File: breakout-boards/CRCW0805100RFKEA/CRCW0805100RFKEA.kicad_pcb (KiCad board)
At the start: 2 copper layers, 21.5 x 38.2 mm, 16 parts, among them J1 Conn_01x12, J2 Conn_01x12

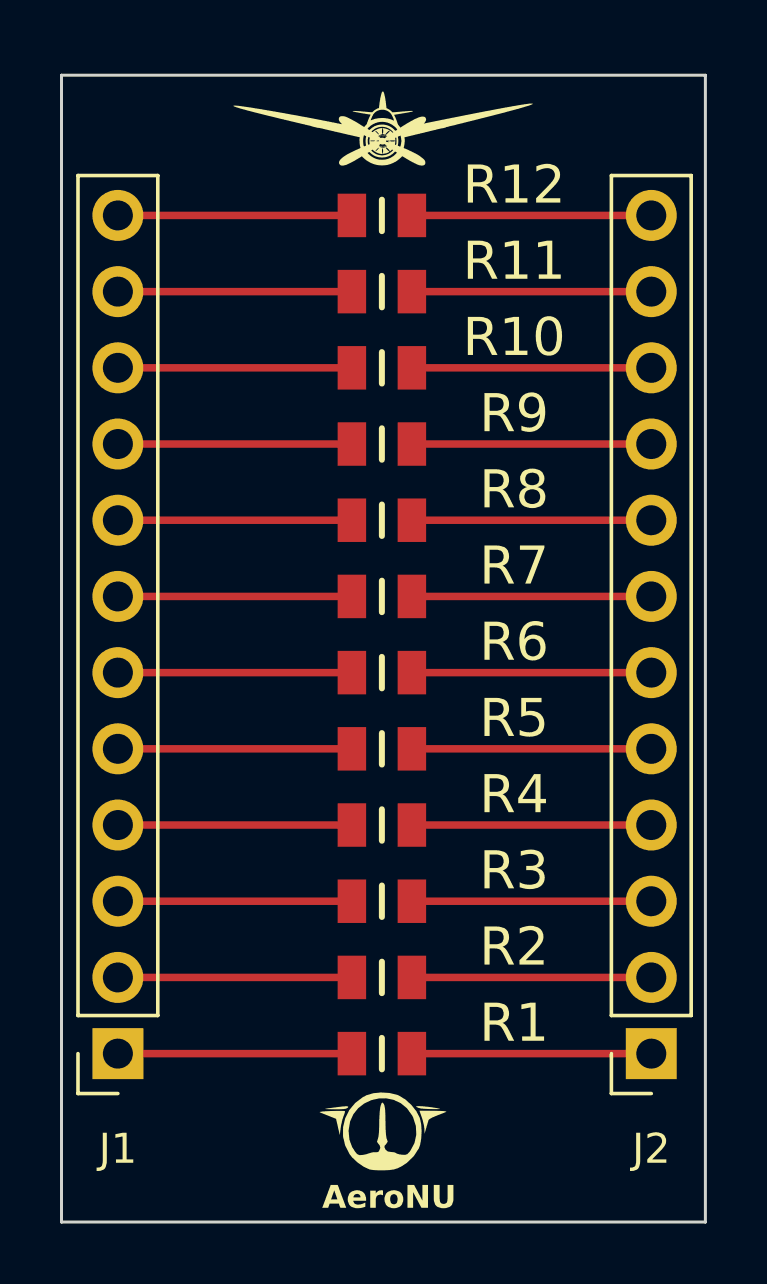
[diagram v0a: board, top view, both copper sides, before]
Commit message: feat: finalize 100ohm board design
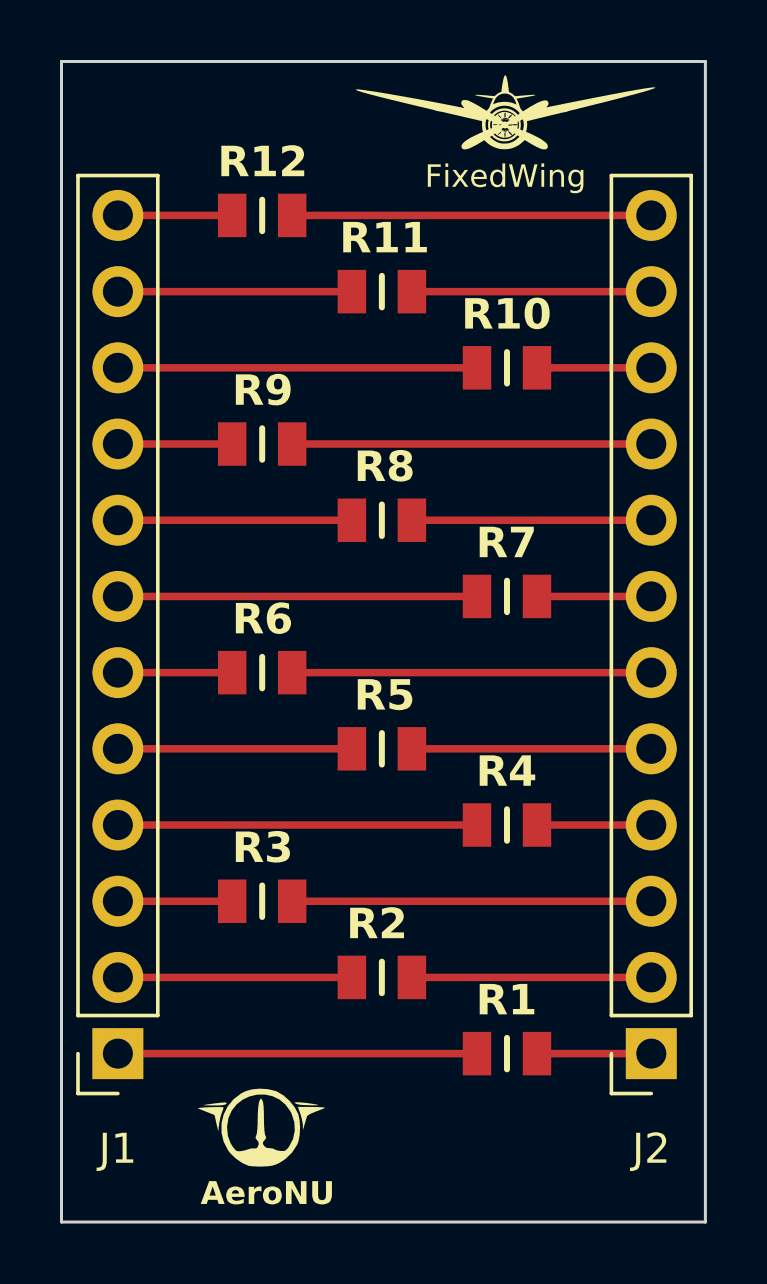
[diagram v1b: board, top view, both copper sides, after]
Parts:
- moved R1 4.17 mm to (165.4, 104.1)
- moved R10 4.17 mm to (165.4, 81.3)
- moved R4 4.17 mm to (165.4, 96.5)
- moved R7 4.17 mm to (165.4, 88.9)
- moved FixedWing 4.14 mm to (165.3, 73.2)
- moved AeroNU 4.05 mm to (157.3, 109.4)
- moved R12 3.99 mm to (157.2, 76.2)
- moved R3 3.99 mm to (157.2, 99.1)
- moved R6 3.99 mm to (157.2, 91.4)
- moved R9 3.99 mm to (157.2, 83.8)
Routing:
- net Net-(J2-Pin_7): track 7.98 -> 3.81 mm
- net Net-(J2-Pin_4): track 7.98 -> 3.81 mm
- net Net-(J2-Pin_10): track 7.98 -> 3.81 mm
- net Net-(J2-Pin_1): track 7.98 -> 3.81 mm
- net Net-(J1-Pin_7): track 7.80 -> 12.0 mm
- net Net-(J1-Pin_4): track 7.80 -> 12.0 mm
- net Net-(J1-Pin_10): track 7.80 -> 12.0 mm
- net Net-(J1-Pin_1): track 7.80 -> 12.0 mm
- net Net-(J2-Pin_9): track 7.98 -> 12.0 mm
- net Net-(J2-Pin_6): track 7.98 -> 12.0 mm
- net Net-(J2-Pin_3): track 7.98 -> 12.0 mm
- net Net-(J2-Pin_12): track 7.98 -> 12.0 mm
- net Net-(J1-Pin_9): track 7.80 -> 3.81 mm
- net Net-(J1-Pin_6): track 7.80 -> 3.81 mm
- net Net-(J1-Pin_3): track 7.80 -> 3.81 mm
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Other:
- board size 21.5 x 38.2 mm -> 21.5 x 38.7 mm
